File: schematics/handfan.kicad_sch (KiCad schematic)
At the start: 12 parts, among them J1 4S 40A BMS, J2 Type-C Boost Charger, J3 ESC, J4 DIGISPARK_IO, J5 DIGISPARK_PWR, J6 POTENTIOMETER, M1 Diatone 1408 4000KV, SW1 15A Rocker Switch

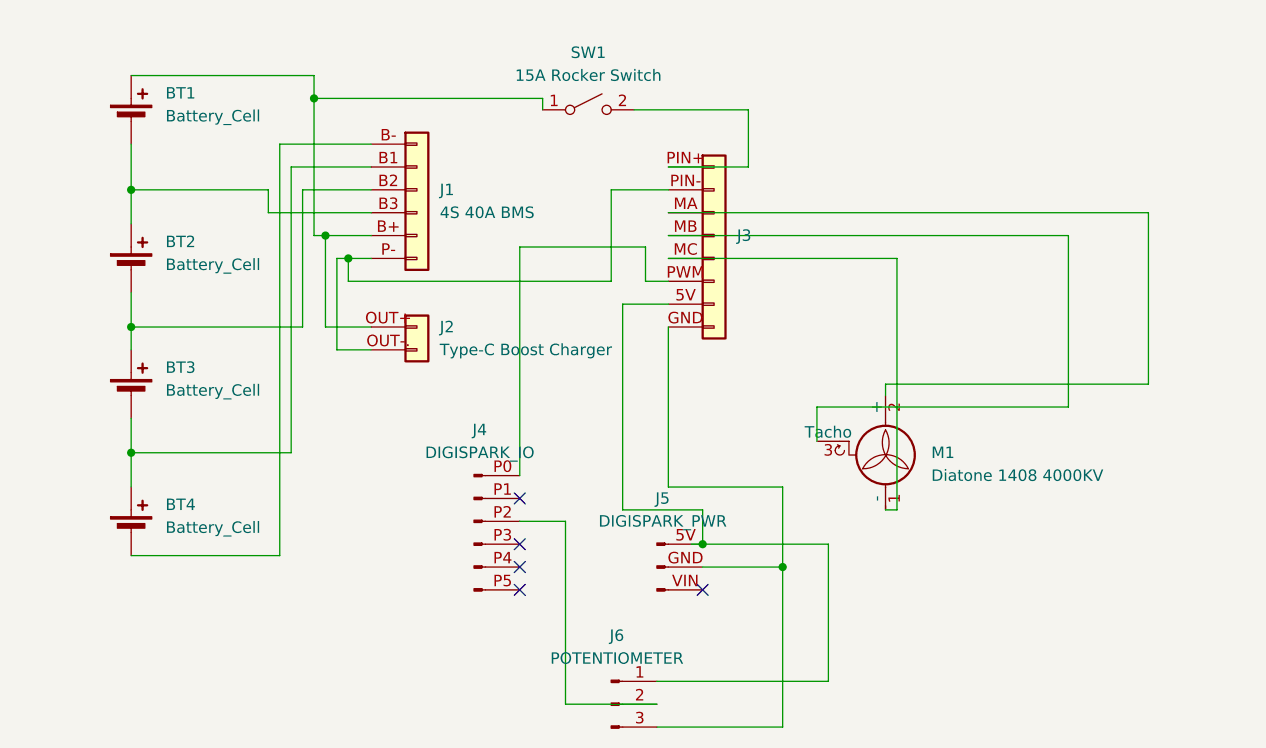
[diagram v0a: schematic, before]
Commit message: changes ask by fabricate
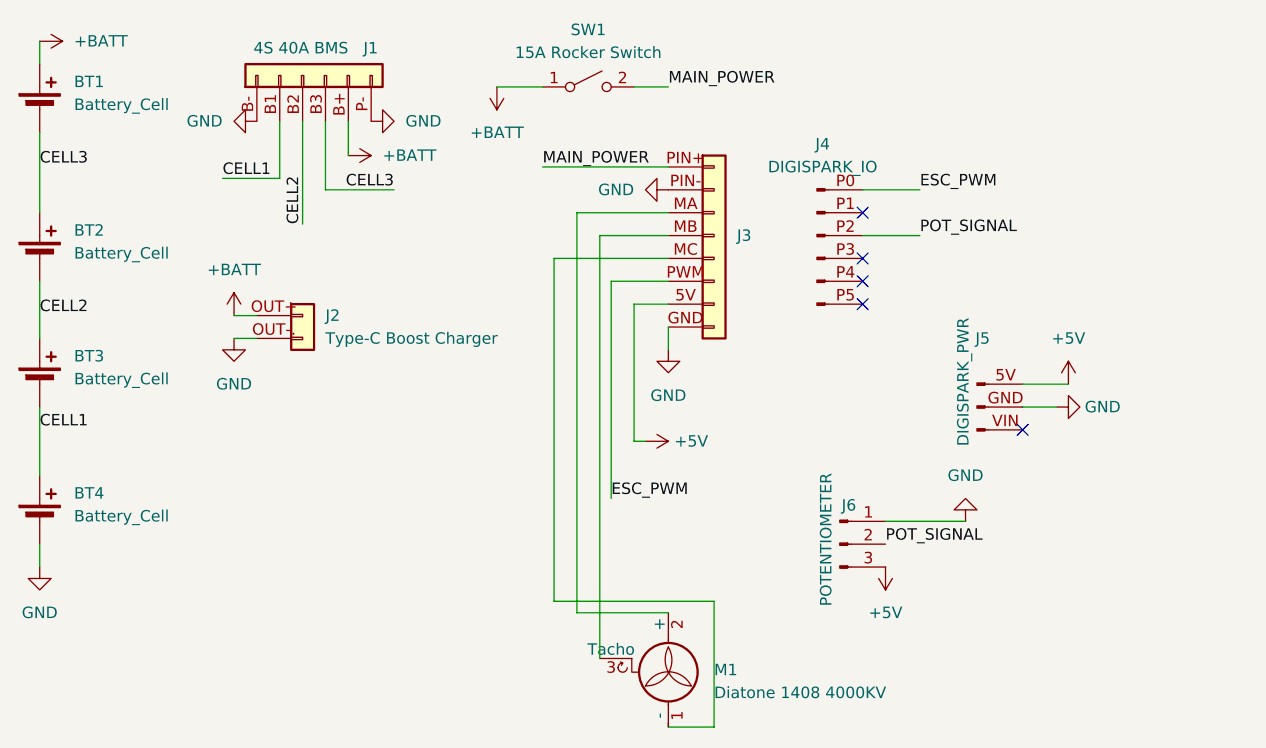
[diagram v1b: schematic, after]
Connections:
- net +5V: now reaches J3.5V (Pin_7), J5.5V (Pin_1)
- net +5V: now also J6.3 (Pin_3); no longer J6.1 (Pin_1)
- net GND: now reaches J3.GND (Pin_8), J5.GND (Pin_2)
- net GND: now also BT4.2 (-), J1.B- (Pin_1), J1.P- (Pin_6), J2.OUT-. (Pin_2), J3.PIN- (Pin_2), J6.1 (Pin_1); no longer J6.3 (Pin_3)
- net MAIN_POWER: now reaches J3.PIN+ (Pin_1), SW1.2 (B)
- net ESC_PWM: now reaches J3.PWM (Pin_6), J4.P0 (Pin_1)
- net +BATT: now reaches BT1.1 (+), J1.B+ (Pin_5), J2.OUT+ (Pin_1), SW1.1 (A)
- net CELL1: now reaches BT3.2 (-), BT4.1 (+), J1.B1 (Pin_2)
- net CELL2: now reaches BT2.2 (-), BT3.1 (+), J1.B2 (Pin_3)
- net CELL3: now reaches BT1.2 (-), BT2.1 (+), J1.B3 (Pin_4)
- net POT_SIGNAL: now reaches J4.P2 (Pin_3), J6.2 (Pin_2)
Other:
- moved on the sheet: BT1, BT2, BT3, BT4, J1, J2, J4, J5, J6, M1, SW1

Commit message: updating
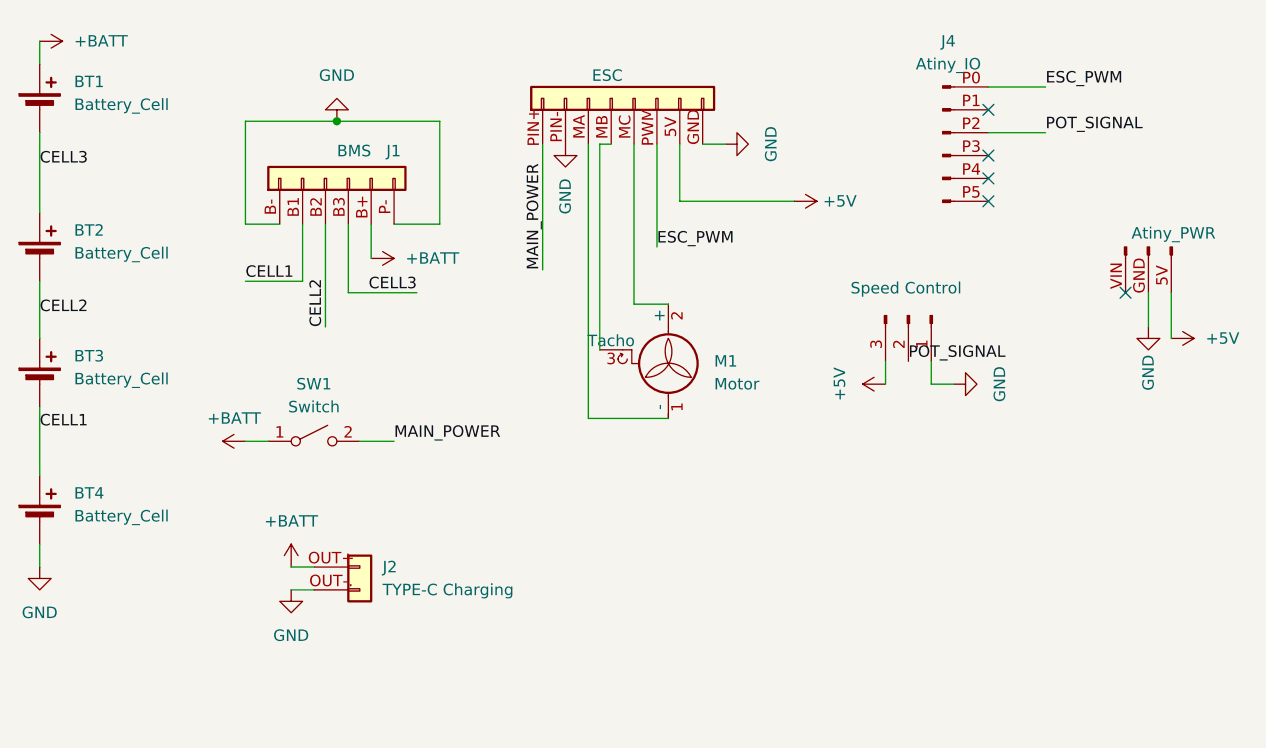
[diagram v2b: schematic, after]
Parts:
- J1: value 4S 40A BMS -> BMS
- J2: value Type-C Boost Charger -> TYPE-C Charging
- J4: value DIGISPARK_IO -> Atiny_IO
- J5: value DIGISPARK_PWR -> Atiny_PWR
- J6: value POTENTIOMETER -> Speed Control
- M1: value Diatone 1408 4000KV -> Motor
- SW1: value 15A Rocker Switch -> Switch
- renumbered J3 to ESC
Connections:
- net at M1.1 (-): now also ESC.MA (Pin_3); no longer ESC.MC (Pin_5)
- net at M1.2 (+): now also ESC.MC (Pin_5); no longer ESC.MA (Pin_3)
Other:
- moved on the sheet: ESC, J1, J2, J4, M1, SW1
